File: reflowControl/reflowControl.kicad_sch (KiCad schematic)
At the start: 12 parts, among them J1 1050170002, U1 MAX6675ISA+, U2 ATmega644PA-A, U3 4N35, U4 MIC5317-3.3xM5, U5 FT231XS, U6 4N35, Y1 Crystal

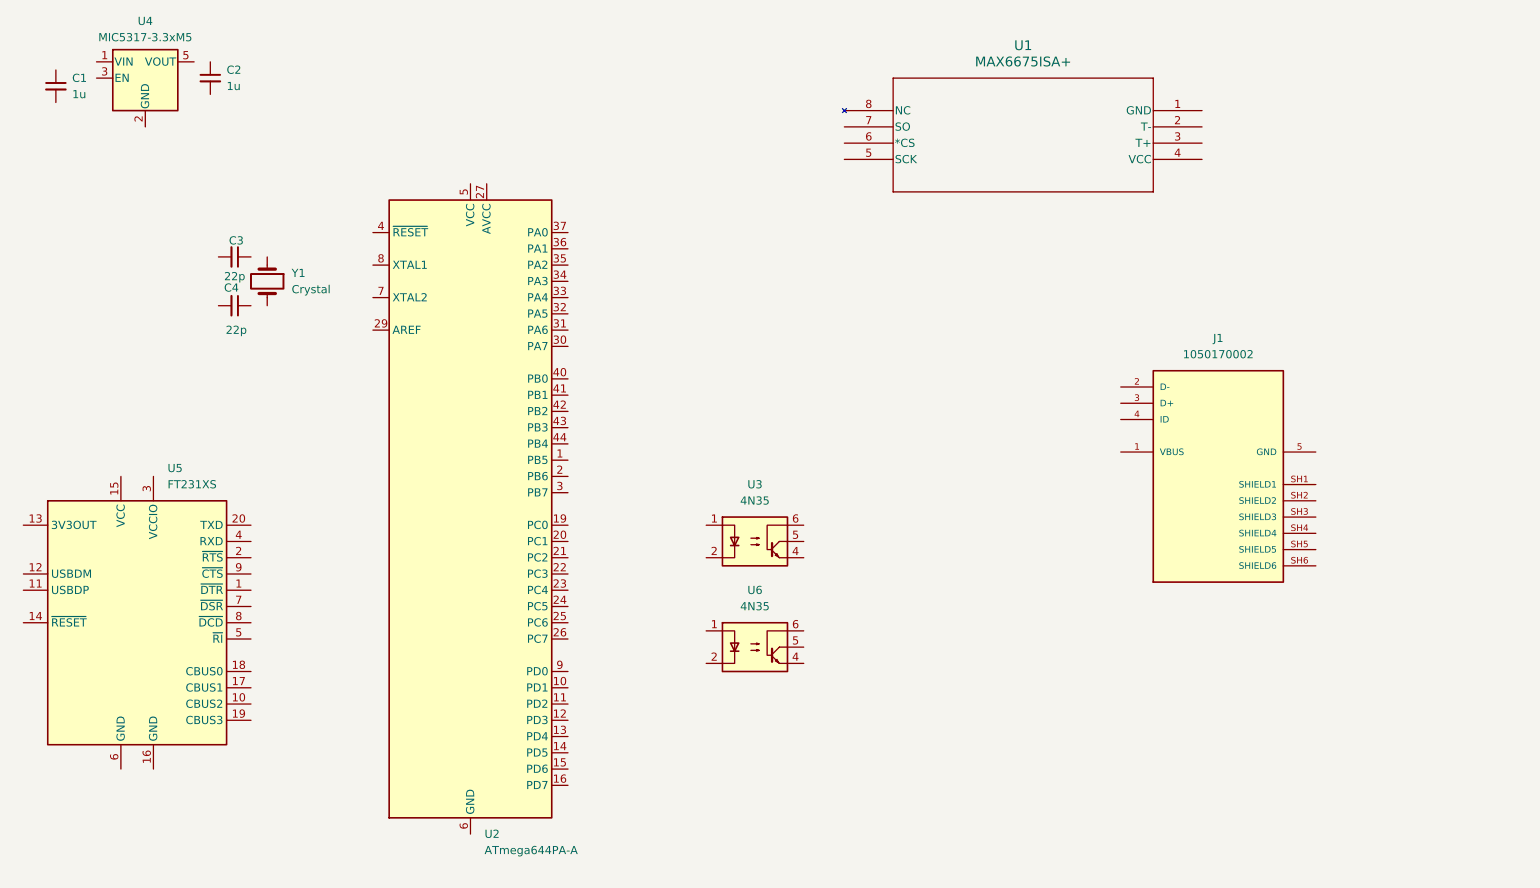
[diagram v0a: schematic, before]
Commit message: schematic work
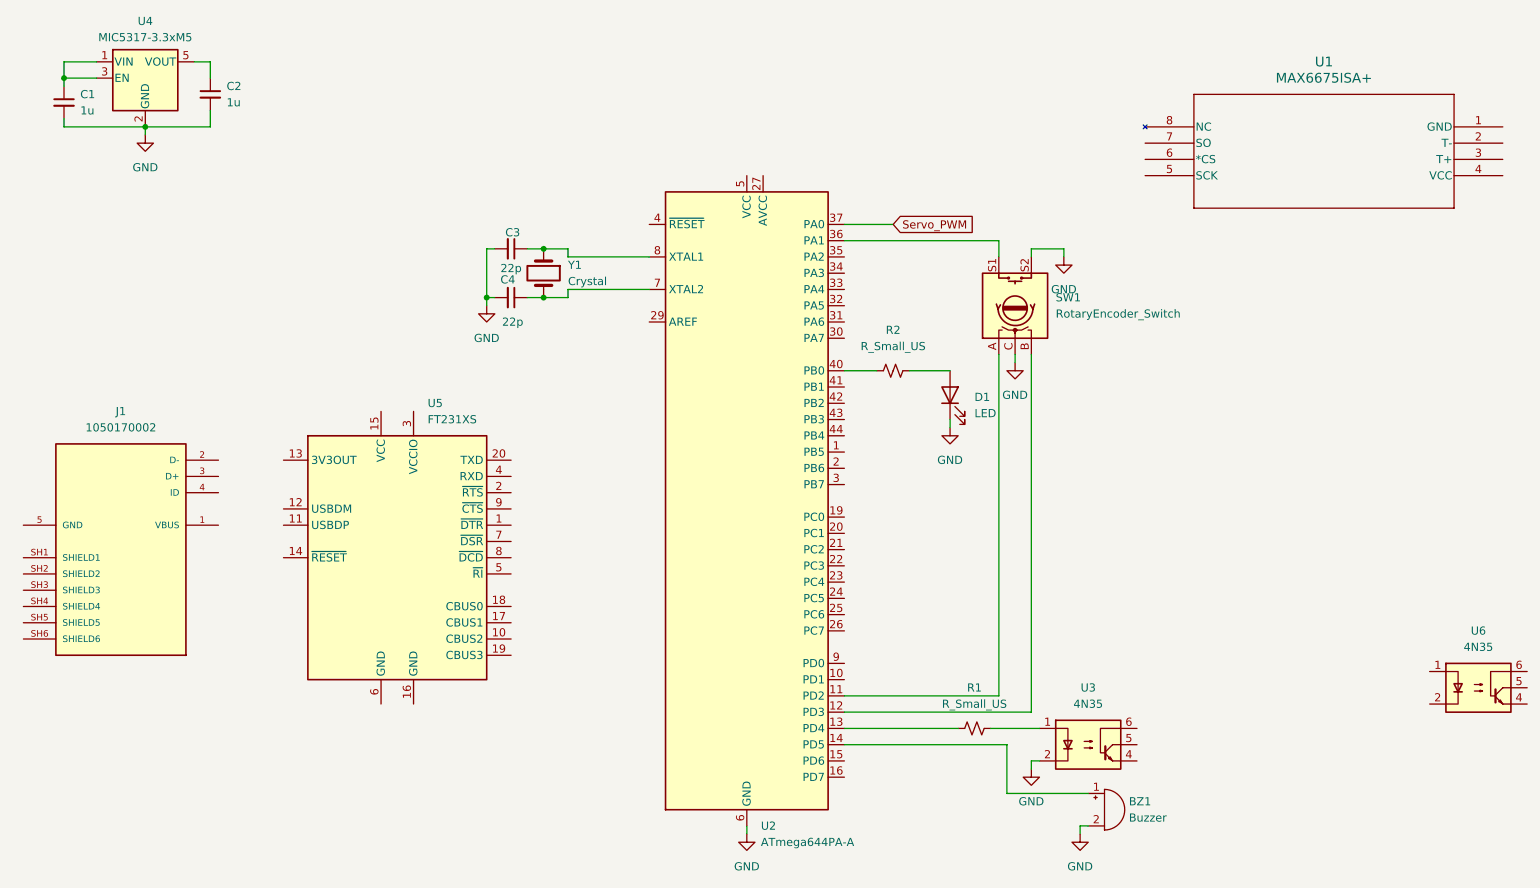
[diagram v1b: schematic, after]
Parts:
- added BZ1: Buzzer, symbol Device:Buzzer
- added D1: LED, symbol Device:LED
- added R1, R2: R_Small_US, symbol Device:R_Small_US
- added SW1: RotaryEncoder_Switch, symbol Device:RotaryEncoder_Switch
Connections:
- net at C3.1: now also U2.8 (XTAL1), Y1.1
- net GND: now reaches C3.2
- net GND: now also C1.2, C2.2, C4.2, U2.18 (GND), U2.28 (GND), U2.39 (GND), U2.6 (GND), U3.2, U4.2 (GND), BZ1.2 (-), D1.1 (K), SW1.C, SW1.S2
- net at U3.1: now also R1.1
- net at C2.1: now also U4.5 (VOUT)
- net at U4.1 (VIN): now also C1.1, U4.3 (EN)
- net at U2.11 (PD2): now also SW1.A
- net at U2.12 (PD3): now also SW1.B
- net at U2.13 (PD4): now also R1.2
- net at U2.14 (PD5): now also BZ1.1 (+)
- net at U2.36 (PA1): now also SW1.S1
- net Servo_PWM: now reaches U2.37 (PA0)
- net at U2.40 (PB0): now also R2.2
- net at U2.7 (XTAL2): now also C4.1, Y1.2
- new net: D1.2 (A), R2.1
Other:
- moved on the sheet: C1, C2, C3, C4, J1, U1, U2, U3, U5, U6, Y1

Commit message: test
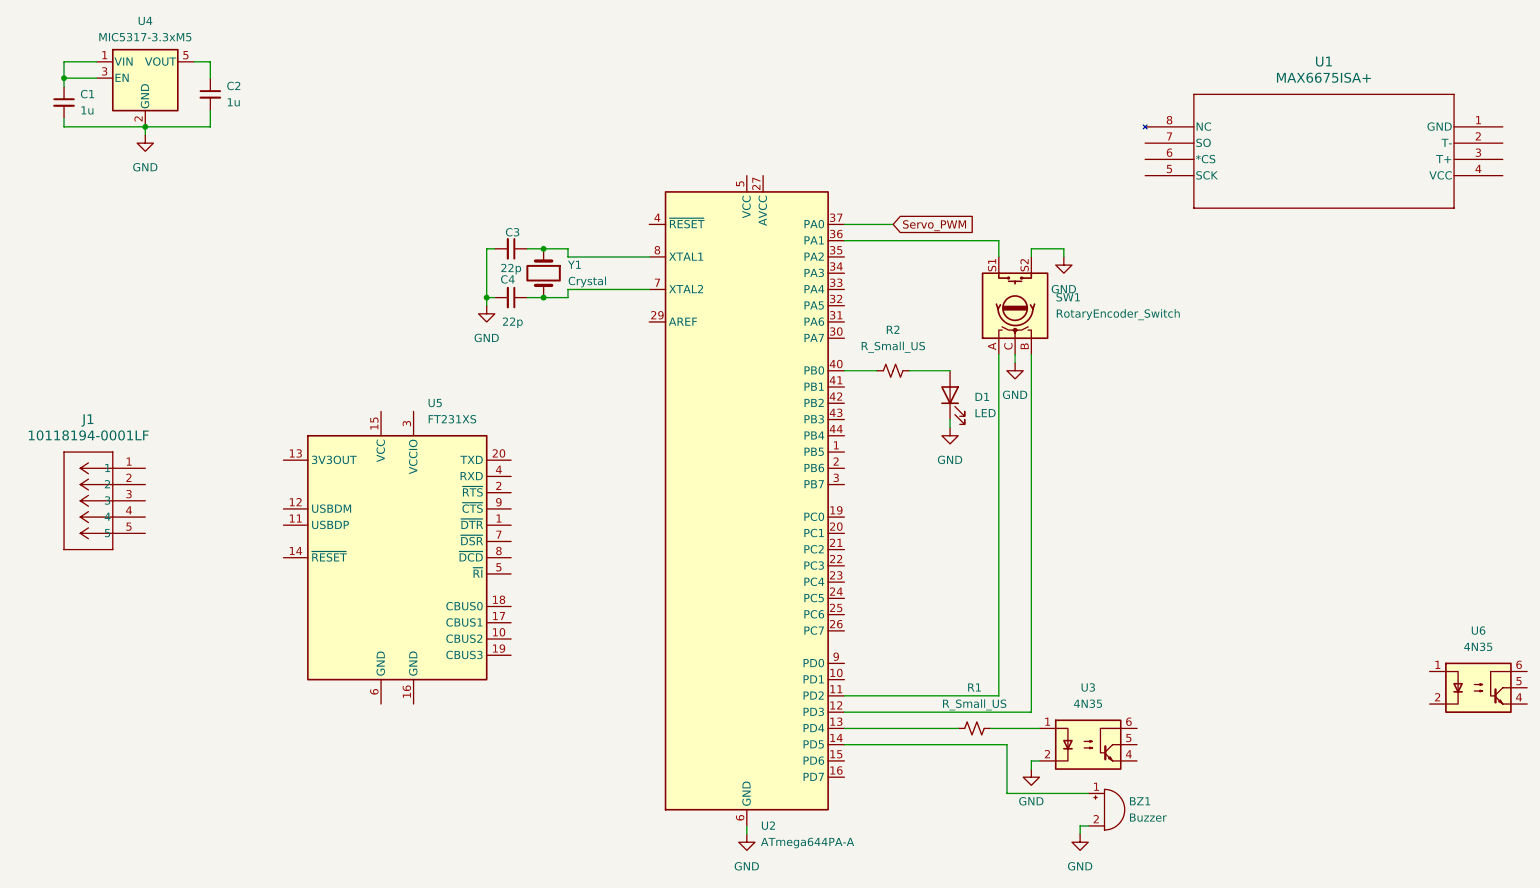
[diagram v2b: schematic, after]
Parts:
- removed J1: 1050170002, localparts:MOLEX_1050170002, symbol 1050170002:1050170002
- added J1: 10118194-0001LF, localparts:CONN_10118194-0001LF_AMP, symbol 2024-05-01_06-00-19:10118194-0001LF
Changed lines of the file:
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@@
+	)
+	(symbol
+		(lib_id "2024-05-01_06-00-19:10118194-0001LF")
+		(at 41.91 90.17 0)
+		(mirror y)
+		(unit 1)
+		(exclude_from_sim no)
+		(in_bom yes)
+		(on_board yes)
+		(dnp no)
+		(fields_autoplaced yes)
+		(property "Reference" "J1"
+			(at 33.02 82.55 0)
+			(effects
+				(font
+					(size 1.524 1.524)
+				)
+			)
+		)
+		(property "Value" "10118194-0001LF"
+			(at 33.02 85.09 0)
+			(effects
+				(font
+					(size 1.524 1.524)
+				)
+			)
+		)
+		(property "Footprint" "localparts:CONN_10118194-0001LF_AMP"
+			(at 41.91 90.17 0)
+			(effects
+				(font
+					(size 1.27 1.27)
+					(italic yes)
+				)
+				(hide yes)
+			)
+		)
+		(property "Datasheet" "10118194-0001LF"
+			(at 41.91 90.17 0)
+			(effects
+				(font
+					(size 1.27 1.27)
+					(italic yes)
+				)
+				(hide yes)
+			)
+		)
+		(property "Description" ""
+			(at 41.91 90.17 0)
+			(effects
+				(font
+					(size 1.27 1.27)
+				)
+				(hide yes)
+			)
+		)
+		(pin "4"
+		)
+		(pin "3"
+		)
+		(pin "5"
+		)
+		(pin "2"
+		)
+		(pin "1"
+		)
+		(instances
+			(project ""
+				(path "/5bc02355-88dd-4e65-870a-598d23d23c1f"
+					(reference "J1")
+					(unit 1)
+				)
+			)
+		)
 	)
 	(symbol
@@
 					(unit 1)
 				)
-			)
-		)
-	)
-	(symbol
-		(lib_id "1050170002:1050170002")
-		(at 38.1 101.6 0)
-		(mirror y)
-		(unit 1)
-		(exclude_from_sim no)
-		(in_bom yes)
-		(on_board yes)
-		(dnp no)
-		(property "Reference" "J1"
-			(at 38.1 81.28 0)
-			(effects
-				(font
-					(size 1.27 1.27)
-				)
-			)
-		)
-		(property "Value" "1050170002"
-			(at 38.1 83.82 0)
-			(effects
-				(font
-					(size 1.27 1.27)
-				)
-			)
-		)
-		(property "Footprint" "localparts:MOLEX_1050170002"
-			(at 38.1 101.6 0)
-			(effects
-				(font
-					(size 1.27 1.27)
-				)
-				(justify bottom)
-				(hide yes)
-			)
-		)
-		(property "Datasheet" ""
-			(at 38.1 101.6 0)
-			(effects
-				(font
-					(size 1.27 1.27)
-				)
-				(hide yes)
-			)
-		)
-		(property "Description" ""
-			(at 38.1 101.6 0)
-			(effects
-				(font
-					(size 1.27 1.27)
-				)
-				(hide yes)
-			)
-		)
-		(property "PARTREV" "B"
-			(at 38.1 101.6 0)
-			(effects
-				(font
-					(size 1.27 1.27)
-				)
-				(justify bottom)
-				(hide yes)
-			)
-		)
-		(property "STANDARD" "Manufacturer Recommendations"
-			(at 38.1 101.6 0)
-			(effects
-				(font
-					(size 1.27 1.27)
-				)
-				(justify bottom)
-				(hide yes)
-			)
-		)
-		(property "OPTION" "MOLEX_CONFIG"
-			(at 38.1 101.6 0)
-			(effects
-				(font
-					(size 1.27 1.27)
-				)
-				(justify bottom)
-				(hide yes)
-			)
-		)
-		(property "MAXIMUM_PACKAGE_HEIGHT" "2.85mm"
-			(at 38.1 101.6 0)
-			(effects
-				(font
-					(size 1.27 1.27)
-				)
-				(justify bottom)
-				(hide yes)
-			)
-		)
-		(property "MANUFACTURER" "Molex"
-			(at 38.1 101.6 0)
-			(effects
-				(font
-					(size 1.27 1.27)
-				)
-				(justify bottom)
-				(hide yes)
-			)
-		)
-		(pin "SH3"
-		)
-		(pin "SH6"
-		)
-		(pin "SH5"
-		)
-		(pin "1"
-		)
-		(pin "4"
-		)
-		(pin "3"
-		)
-		(pin "2"
-		)
-		(pin "SH4"
-		)
-		(pin "SH1"
-		)
-		(pin "SH2"
-		)
-		(pin "5"
-		)
-		(instances
-			(project ""
-				(path "/5bc02355-88dd-4e65-870a-598d23d23c1f"
-					(reference "J1")
-					(unit 1)
-				)
